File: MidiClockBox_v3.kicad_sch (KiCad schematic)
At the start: 87 parts, among them J1 Midi In 0, J10 Display, J11 Midi Out 3, J12 Midi Out 4, J13 Midi Out 5, J14 Sync Out 0, J15 Sync Out 1, J16 Spare, J17 Conn_01x07, J18 Conn_01x07, J2 ICSP, J3 WS2812, J4 Conn_02x07_Odd_Even, J5 Conn_02x12_Counter_Clockwise, J6 Midi Out 0, J7 Midi Out 1, J8 Midi Out 2, J9 WS2812, SW1 RotaryEncoder_Switch, SW2 TAP, SW3 Start, SW4 Stop, SW5 Preset1, SW6 Preset2, SW7 Preset3, U1 CD74HC4067SM, U2 74LS241, U3 6N138, U4 74HC595, U6 74LS08, U7 74LS08, U8 74HC595, U9 74LS241

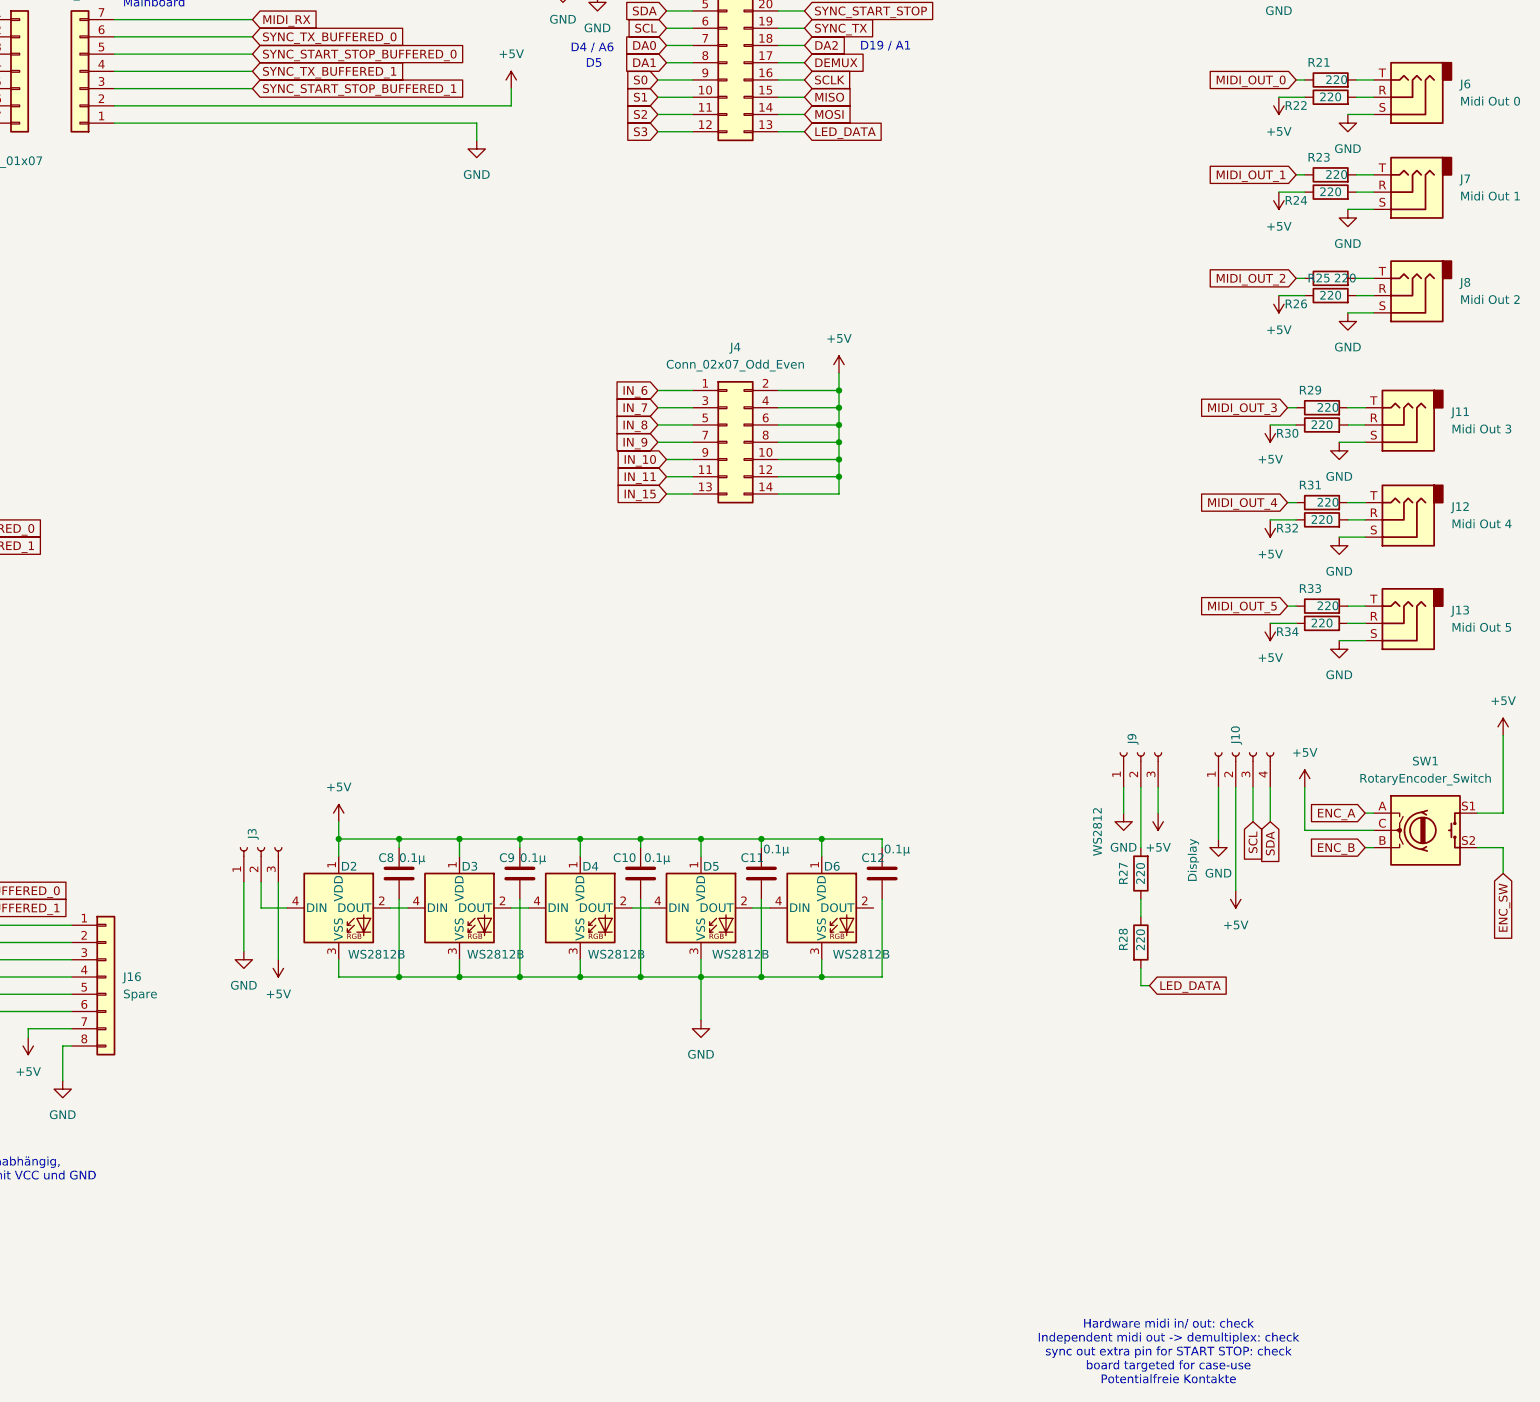
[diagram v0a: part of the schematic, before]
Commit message: pcb looks complete
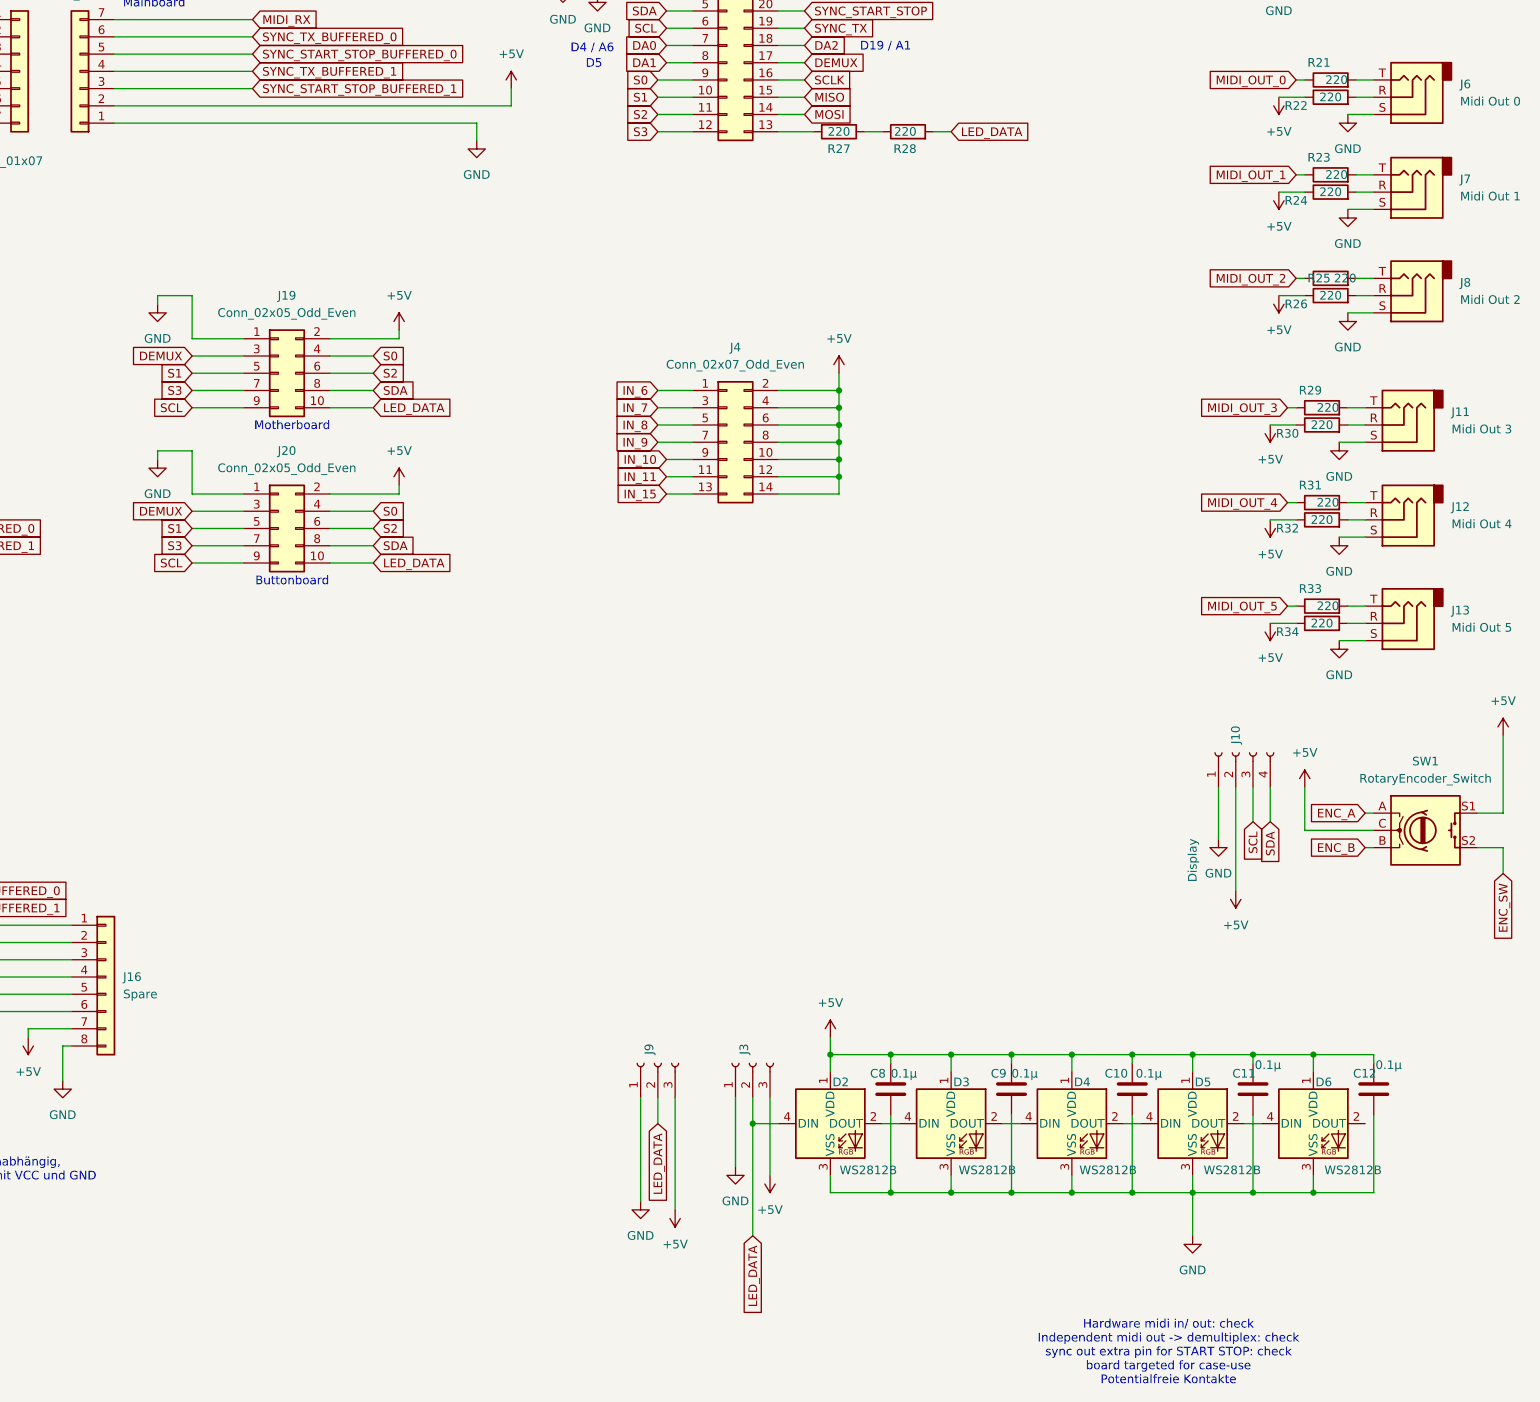
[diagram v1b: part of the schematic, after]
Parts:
- added J19, J20: Conn_02x05_Odd_Even, Connector_PinHeader_2.54mm:PinHeader_2x05_P2.54mm_Vertical, symbol Connector_Generic:Conn_02x05_Odd_Even
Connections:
- net +5V: now also J19.2 (Pin_2), J20.2 (Pin_2)
- net DEMUX: now also J19.3 (Pin_3), J20.3 (Pin_3)
- net GND: now also J19.1 (Pin_1), J20.1 (Pin_1)
- net LED_DATA: now also D2.4 (DIN), J3.2 (Pin_2), J9.2 (Pin_2), J19.10 (Pin_10), J20.10 (Pin_10); no longer J5.13 (Pin_13)
- net S0: now also J19.4 (Pin_4), J20.4 (Pin_4)
- net S1: now also J19.5 (Pin_5), J20.5 (Pin_5)
- net S2: now also J19.6 (Pin_6), J20.6 (Pin_6)
- net S3: now also J19.7 (Pin_7), J20.7 (Pin_7)
- net SCL: now also J19.9 (Pin_9), J20.9 (Pin_9)
- net SDA: now also J19.8 (Pin_8), J20.8 (Pin_8)
- net at R27.2: now also J5.13 (Pin_13); no longer J9.2 (Pin_2)
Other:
- note added: "Buttonboard"
- note added: "Motherboard"
- moved on the sheet: C10, C11, C12, C8, C9, D2, D3, D4, D5, D6, J3, R27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
